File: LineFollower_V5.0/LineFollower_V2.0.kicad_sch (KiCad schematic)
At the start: 19 parts, among them J1 BAT, J2 Conn_01x05, J3 ICSP, J4 Conn_01x06_MountingPin, J5 Conn_01x10, J6 MotA, J7 MotB, SW1 RESET, SW2 SW_SPDT, U1 ATmega328P-AU, U2 LM78L05_TO92, U3 TB6612FNG, Y1 20MHz

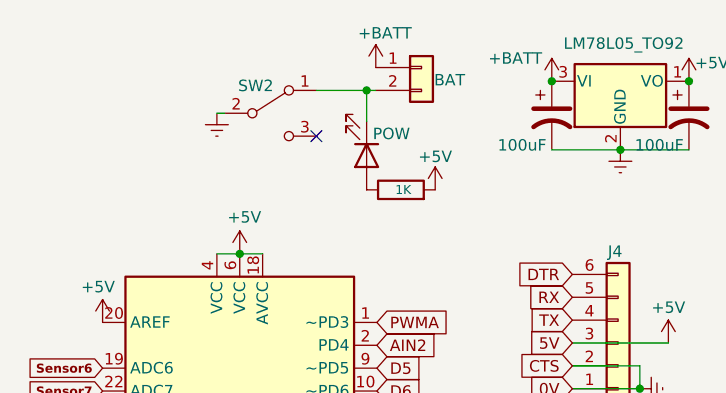
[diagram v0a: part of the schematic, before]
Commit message: f
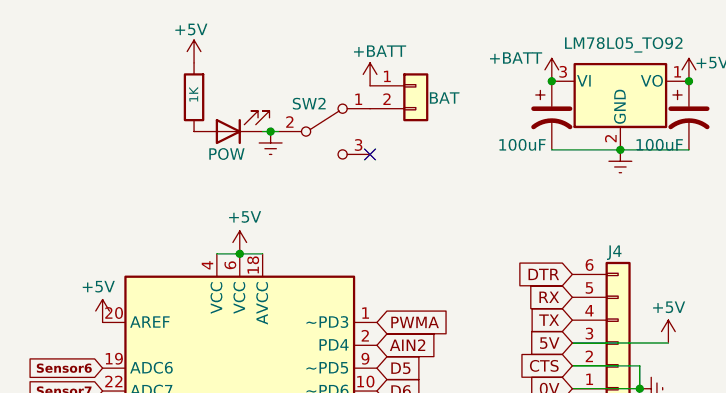
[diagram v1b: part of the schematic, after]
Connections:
- net Earth: now also D1.1 (K)
- net at J1.2 (Pin_2), SW2.1 (A): no longer D1.1 (K)
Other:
- moved on the sheet: SW2
